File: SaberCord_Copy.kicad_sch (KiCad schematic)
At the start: 2 parts, among them J1 Conn_02x07_Counter_Clockwise, J2 Conn_02x12_Row_Letter_Last

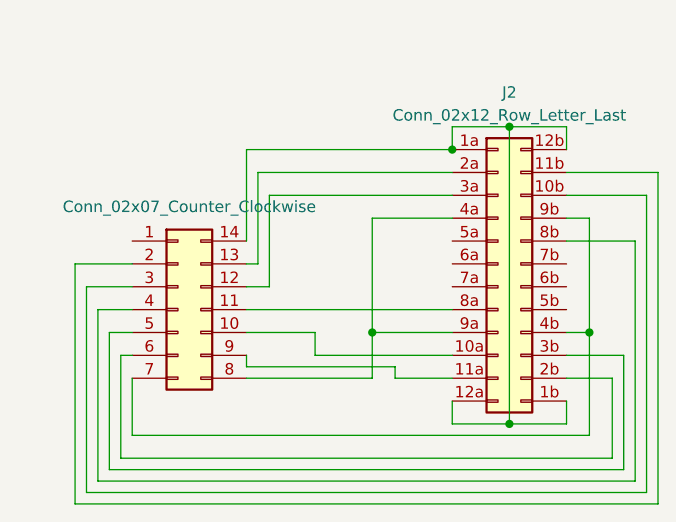
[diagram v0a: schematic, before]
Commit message: refine footprint and schema
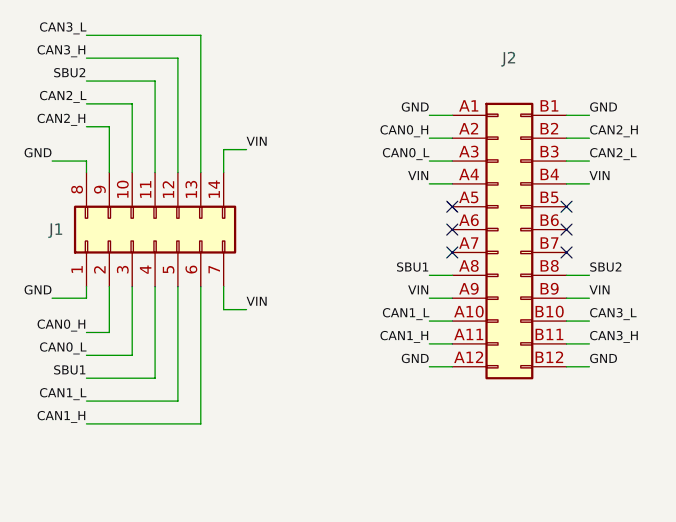
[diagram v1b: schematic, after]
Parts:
- removed J1: Conn_02x07_Counter_Clockwise, symbol Connector_Generic:Conn_02x07_Counter_Clockwise
- removed J2: Conn_02x12_Row_Letter_Last, symbol USB_C_24P_Lettered:Conn_02x12_Row_Letter_Last
- added J1: Conn_02x07_Row_Letter_Last, CommaPogo_Library:2x7_Pogo_Male, symbol Connector_Generic:Conn_02x07_Row_Letter_Last
- added J2: Conn_02x12_Row_Letter_Last, CommaPogo_Library:GCT_USB4056-03-A_REVA2, symbol Connector_Generic:Conn_02x12_Row_Letter_Last
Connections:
- new net CAN0_H: J1.2 (Pin_2a), J2.A2 (a2)
- new net CAN0_L: J1.3 (Pin_3a), J2.A3 (a3)
- new net CAN1_H: J1.6 (Pin_6a), J2.A11 (a11)
- new net CAN1_L: J1.5 (Pin_5a), J2.A10 (a10)
- new net CAN2_H: J1.9 (Pin_2b), J2.B2 (b2)
- new net CAN2_L: J1.10 (Pin_3b), J2.B3 (b3)
- new net CAN3_H: J1.12 (Pin_5b), J2.B11 (b11)
- new net CAN3_L: J1.13 (Pin_6b), J2.B10 (b10)
- new net GND: J1.1 (Pin_1a), J1.8 (Pin_1b), J2.A1 (a1), J2.A12 (a12), J2.B1 (b1), J2.B12 (b12)
- new net SBU1: J1.4 (Pin_4a), J2.A8
- new net SBU2: J1.11 (Pin_4b), J2.B8 (b8)
- new net VIN: J1.14 (Pin_7b), J1.7 (Pin_7a), J2.A4 (a4), J2.A9 (a9), J2.B4 (b4), J2.B9 (b9)
- no-connect marks 0 -> 6
